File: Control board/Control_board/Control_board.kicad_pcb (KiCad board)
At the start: 2 copper layers, 146.8 x 119 mm, 84 parts, among them J1 KEYPAD, J2 UART_conn, J3 Power_IN, J4 SPI_conn, J5 Triac Control, J6 MDB, SW1 RESET, SW2 Button1, SW3 Button2, T1 BCX17, T2 BCX17, U1 AT45DB321E-SHF-T, U10 SP3485EN, U11 Debug, U12 PCA9554AD_118, U13 LM317DCY, U2 LM2576HVS-5, U3 LoRa, U4 Wifi, U6 STM32F103C8Tx, U7 RTC_DS3234, U8 DS3232SN-T&R, U9 OLED, Y1 8MHZ

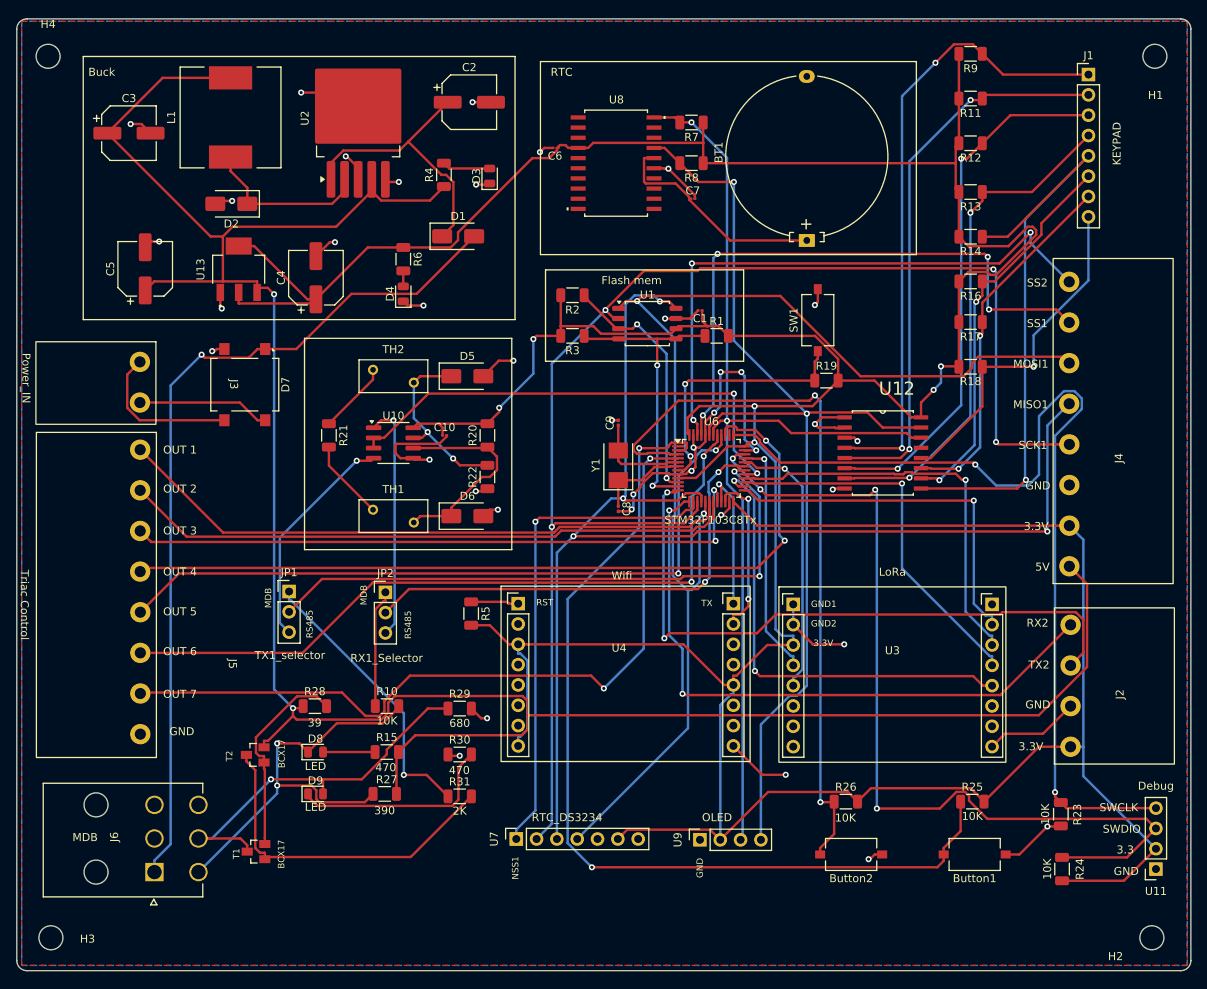
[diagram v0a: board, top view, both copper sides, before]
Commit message: last update
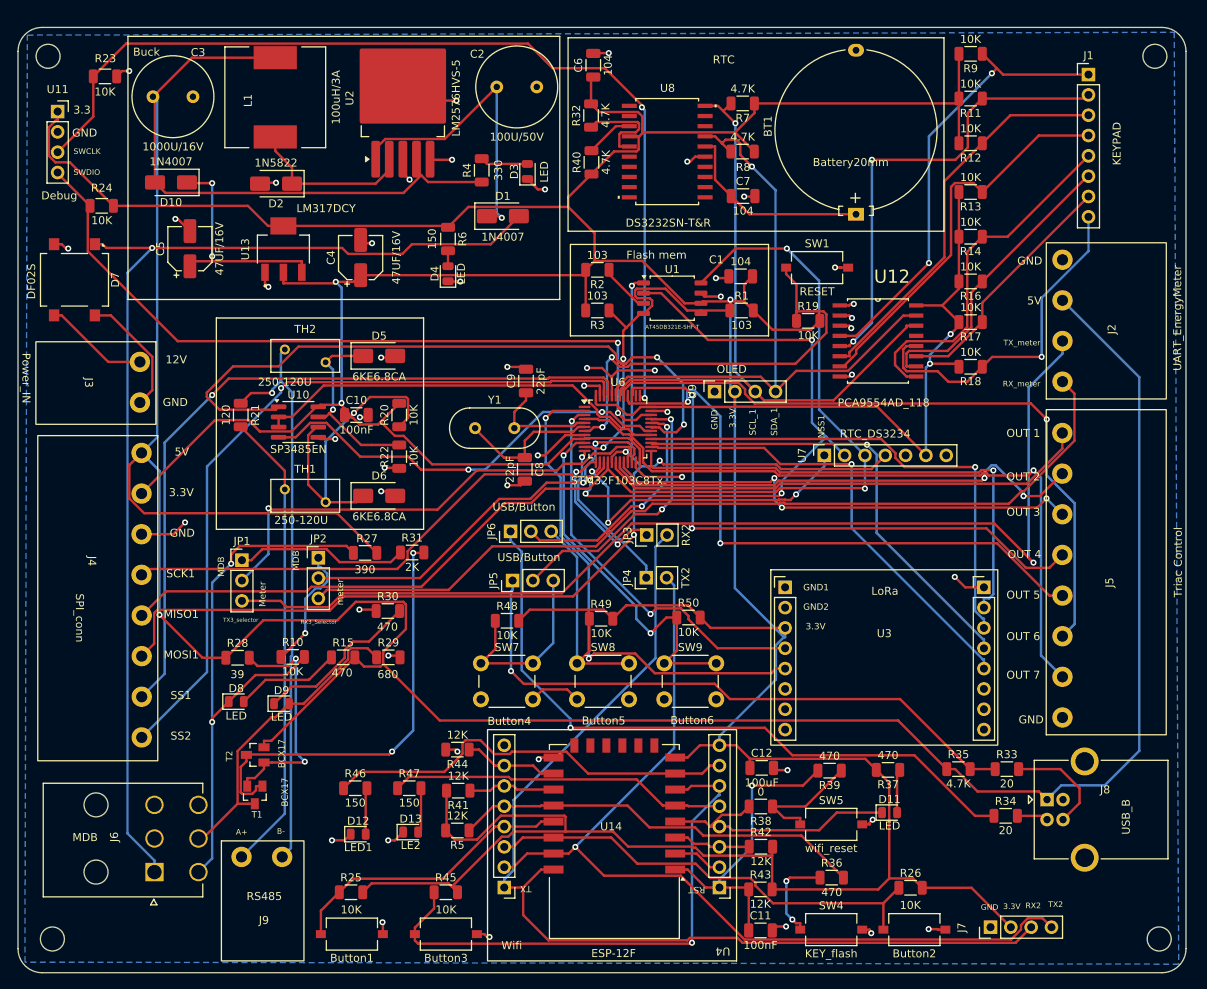
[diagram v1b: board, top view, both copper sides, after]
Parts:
- added C11: 100nF, Capacitor_SMD:C_1206_3216Metric, F.Cu at (155.0, 155.2)
- added C12: 100uF, Capacitor_SMD:C_1206_3216Metric, F.Cu at (155.2, 134.9)
- added D10: 1N4007, Diode_SMD:D_SMA, F.Cu at (81.3, 61.7)
- added D11: LED, LED_SMD:LED_0805_2012Metric, F.Cu at (171.2, 140.5)
- added D12: LED1, LED_SMD:LED_0805_2012Metric, F.Cu at (104.8, 143.2)
- added D13: LE2, LED_SMD:LED_0805_2012Metric, F.Cu at (111.3, 143.0)
- added J7: UART_wifi, Connector_PinHeader_2.54mm:PinHeader_1x04_P2.54mm_Vertical, F.Cu at (183.8, 154.8)
- added J8: USB_B, Connector_USB:USB_B_OST_USB-B1HSxx_Horizontal, F.Cu at (190.9, 138.9)
- added J9: RS485, smart_meter:RC2, F.Cu at (92.9, 139.4)
- added JP3: RX2, Connector_PinHeader_2.54mm:PinHeader_1x02_P2.54mm_Vertical, F.Cu at (140.8, 105.8)
- added JP4: TX2, Connector_PinHeader_2.54mm:PinHeader_1x02_P2.54mm_Vertical, F.Cu at (140.8, 111.2)
- added JP5: USB/Button, Connector_PinHeader_2.54mm:PinHeader_1x03_P2.54mm_Vertical, F.Cu at (124.1, 111.5)
- added JP6: USB/Button, Connector_PinHeader_2.54mm:PinHeader_1x03_P2.54mm_Vertical, F.Cu at (123.8, 105.4)
- added R32: 4.7K, Resistor_SMD:R_1206_3216Metric, F.Cu at (133.9, 53.4)
- added R33: 20, Resistor_SMD:R_1206_3216Metric, F.Cu at (185.8, 135.1)
- added R34: 20, Resistor_SMD:R_1206_3216Metric, F.Cu at (185.7, 140.9)
- added R35: 4.7K, Resistor_SMD:R_1206_3216Metric, F.Cu at (179.8, 135.1)
- added R36: 470, Resistor_SMD:R_1206_3216Metric, F.Cu at (163.9, 148.6)
- added R37: 470, Resistor_SMD:R_1206_3216Metric, F.Cu at (171.0, 135.2)
- added R38: 0, Resistor_SMD:R_1206_3216Metric, F.Cu at (155.1, 139.8)
- added R39: 470, Resistor_SMD:R_1206_3216Metric, F.Cu at (163.7, 135.3)
- added R40: 4.7K, Resistor_SMD:R_1206_3216Metric, F.Cu at (133.9, 59.2)
- added R41: 12K, Resistor_SMD:R_1206_3216Metric, F.Cu at (117.3, 137.8)
- added R42: 12K, Resistor_SMD:R_1206_3216Metric, F.Cu at (155.1, 144.8)
- added R43: 12K, Resistor_SMD:R_1206_3216Metric, F.Cu at (155.0, 150.1)
- added R44: 12K, Resistor_SMD:R_1206_3216Metric, F.Cu at (117.2, 132.6)
- added R45: 10K, Resistor_SMD:R_1206_3216Metric, F.Cu at (115.7, 150.5)
- added R46: 150, Resistor_SMD:R_1206_3216Metric, F.Cu at (104.4, 137.5)
- added R47: 150, Resistor_SMD:R_1206_3216Metric, F.Cu at (111.1, 137.5)
- added R48: 10K, Resistor_SMD:R_1206_3216Metric, F.Cu at (123.4, 116.5)
- added R49: 10K, Resistor_SMD:R_1206_3216Metric, F.Cu at (135.1, 116.3)
- added R50: 10K, Resistor_SMD:R_1206_3216Metric, F.Cu at (146.0, 116.1)
- added SW4: KEY_flash, Button_Switch_SMD:SW_Tactile_SPST_NO_Straight_CK_PTS636Sx25SMTRLFS, F.Cu at (163.9, 155.1)
- added SW5: wifi_reset, Button_Switch_SMD:SW_Tactile_SPST_NO_Straight_CK_PTS636Sx25SMTRLFS, F.Cu at (163.9, 142.0)
- added SW6: Button3, Button_Switch_SMD:SW_Tactile_SPST_NO_Straight_CK_PTS636Sx25SMTRLFS, F.Cu at (115.7, 155.7)
- added SW7: Button4, Button_Switch_THT:SW_PUSH_6mm, F.Cu at (120.1, 121.9)
- added SW8: Button5, Button_Switch_THT:SW_PUSH_6mm, F.Cu at (132.1, 121.9)
- added SW9: Button6, Button_Switch_THT:SW_PUSH_6mm, F.Cu at (143.0, 121.9)
- added U14: ESP-12F, RF_Module:ESP-12E, F.Cu at (136.8, 144.1)
- C1, C10, C6, C7: footprint Capacitor_SMD:C_01005_0402Metric -> Capacitor_SMD:C_1206_3216Metric
- C2, C3: footprint Capacitor_SMD:CP_Elec_6.3x7.7 -> Capacitor_THT:C_Radial_D10.0mm_H12.5mm_P5.00mm
- C4, C5: footprint Capacitor_SMD:CP_Elec_6.3x7.7 -> Capacitor_SMD:CP_Elec_5x5.3
- C8, C9: footprint Capacitor_SMD:C_0201_0603Metric -> Capacitor_SMD:C_1206_3216Metric
- J2: value UART_conn -> UART_EnergyMeter
- JP1: value TX1_selector -> TX3_selector
- JP2: value RX1_Selector -> RX3_Selector
- R1, R2, R3: value 10K -> 103
- R5: value 10K -> 12K
- Y1: footprint Crystal:Crystal_SMD_5032-2Pin_5.0x3.2mm -> Crystal:Crystal_HC18-U_Vertical
- moved U11 166.8 mm to (67.2, 52.9), turned to 0 degrees
- moved R23 150.9 mm to (73.1, 48.5), turned to 0 degrees
- moved R24 145.9 mm to (72.7, 64.7), turned to 0 degrees
- moved J4 103.4 mm to (85.9, 116.6), turned to -90 degrees
- moved J5 99.2 mm to (184.6, 107.6), turned to 90 degrees
- moved R25 78.5 mm to (103.9, 150.5)
- moved SW2 78.5 mm to (104.0, 155.7)
- moved U7 61.5 mm to (163.0, 95.9)
- moved U9 56.1 mm to (149.3, 87.9)
- moved U4 53.6 mm to (137.1, 158.9), turned to 180 degrees
- moved J2 45.6 mm to (184.2, 79.3)
- moved R31 31.1 mm to (111.5, 108.0)
- moved R27 30.2 mm to (105.6, 108.1)
- moved R5 27.2 mm to (117.1, 142.7), turned to 180 degrees
- moved D7 25.0 mm to (69.3, 73.9)
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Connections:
- C5 pad 1: /5V -> Net-(D10-K)
- J2 pad 1: /3.3V -> /RX_Meter
- J2 pad 2: /GND -> /TX_Meter
- J2 pad 3: /TX2 -> /5V
- J2 pad 4: /RX2 -> /GND
- J5 pad 1: /OUT1 -> /GND
- J5 pad 2: /OUT2 -> /OUT7
- J5 pad 3: /OUT3 -> /OUT6
- J5 pad 4: /OUT4 -> /OUT5
- J5 pad 5: /OUT5 -> /OUT4
- J5 pad 6: /OUT6 -> /OUT3
- J5 pad 7: /OUT7 -> /OUT2
- J5 pad 8: /GND -> /OUT1
- JP1 pad 2: /TX1 -> /TX3
- JP1 pad 3: /TX_485 -> /TX_Meter
- JP2 pad 2: /RX1 -> /RX3
- JP2 pad 3: /RX_485 -> /RX_Meter
- R2 pad 1: /RST_flash -> Net-(U1-~{RESET})
- R5 pad 1: /RST_WIFI -> /GPIO0
- U1 pad 3: /RST_flash -> Net-(U1-~{RESET})
- U10 pad 1: /RX_485 -> /RX1
- U10 pad 4: /TX_485 -> /TX1
- U11 pad 1: /GND -> /3.3V
- U11 pad 2: /3.3V -> /GND
- U11 pad 3: /SWDIO -> /SWCLK
- U11 pad 4: /SWCLK -> /SWDIO
- U13 pad 3: /5V -> Net-(D10-K)
- U4 pad ADC: unconnected-(U4-PadADC) -> /ADC
- U4 pad CH_PC: /3.3V -> /EN
- U4 pad GPIO0: /3.3V -> /GPIO0
- U4 pad GPIO12: unconnected-(U4-PadGPIO12) -> /Button3
- U4 pad GPIO13: unconnected-(U4-PadGPIO13) -> /LED 1
- U4 pad GPIO14: unconnected-(U4-PadGPIO14) -> /LED 2
- U4 pad GPIO15: /GND -> /GPIO15
- U4 pad GPIO16: unconnected-(U4-PadGPIO16) -> /GPIO16
- U4 pad GPIO2: unconnected-(U4-PadGPIO2) -> /GPIO2
- U4 pad GPIO4: unconnected-(U4-PadGPIO4) -> /Button1
- U4 pad GPIO5: unconnected-(U4-PadGPIO5) -> /Button2
- U4 pad RX: /RX3 -> /TX2
- U4 pad TX: /TX3 -> /RX2
- U6 pad 10: /RST_flash -> /Button6
- U6 pad 12: /TX2 -> /TX2_stm
- U6 pad 13: /RX2 -> /RX2_stm
- U6 pad 2: /Button1 -> /DIO0
- U6 pad 3: /Button2 -> /RST_LoRa
- U6 pad 32: /DIO0 -> /PA11
- U6 pad 33: /RST_LoRa -> /PA12
- U8 pad 3: unconnected-(U8-32KHZ-Pad3) -> Net-(U8-32KHZ)
- U8 pad 5: unconnected-(U8-*INT/SQW-Pad5) -> Net-(U8-*INT/SQW)
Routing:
- net /TX_Meter: track 0.00 -> 135.3 mm, vias 0 -> 1
- net /RX_Meter: track 0.00 -> 110.8 mm
- net /5V: track 299.3 -> 409.5 mm, vias 2 -> 1
- net /3.3V: track 588.2 -> 697.8 mm, vias 6 -> 5
- net /USB_DM: track 0.00 -> 85.1 mm, vias 0 -> 1
- net /Button1: track 118.1 -> 36.6 mm, vias 2 -> 0
- net /USB_DP: track 0.00 -> 77.0 mm, vias 0 -> 1
- net /Button3: track 0.00 -> 68.7 mm, vias 0 -> 1
- net /B-: track 9.01 -> 71.1 mm, vias 0 -> 1
- net /LED 1: track 0.00 -> 52.6 mm
- net /GPIO0: track 0.00 -> 51.8 mm
- net /RX2: track 78.8 -> 129.1 mm, vias 2 -> 0
- net /A+: track 10.1 -> 58.3 mm
- net /Button6: track 0.00 -> 47.0 mm, vias 0 -> 2
- net /SDA_1: track 129.7 -> 83.2 mm, vias 2 -> 1
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- removed copper zone on F.Cu, net /GND
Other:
- board size 146.8 x 119 mm -> 146 x 118.2 mm
- board text added: "12V"
- board text added: "A+"
- board text added: "B-"
- board text added: "Meter"
- board text added: "RX_meter"
- board text added: "SCL_1"
- board text added: "SDA_1"
- board text added: "TX_meter"
- board text added: "meter"
- board text removed: "RS485"
